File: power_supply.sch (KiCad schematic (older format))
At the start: 12 parts, among them IC704 TPS82085, IC705 TPS82085

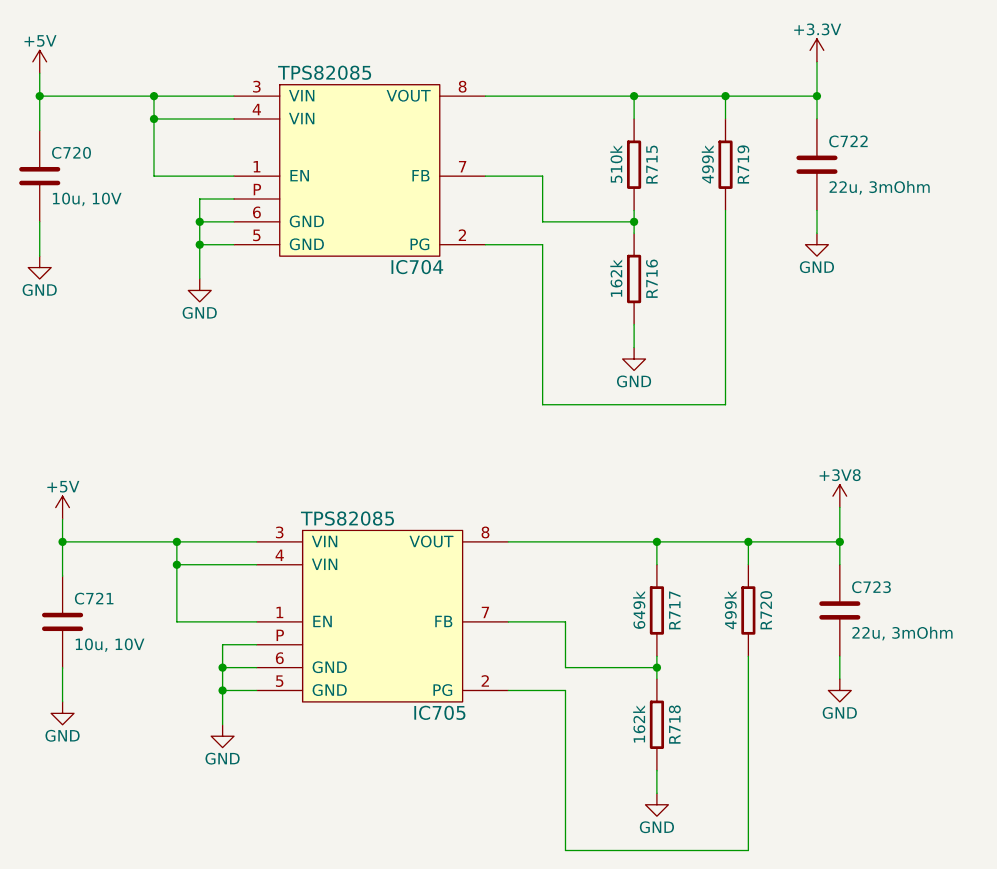
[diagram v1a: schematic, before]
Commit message: power Sypply for Tobyfinish
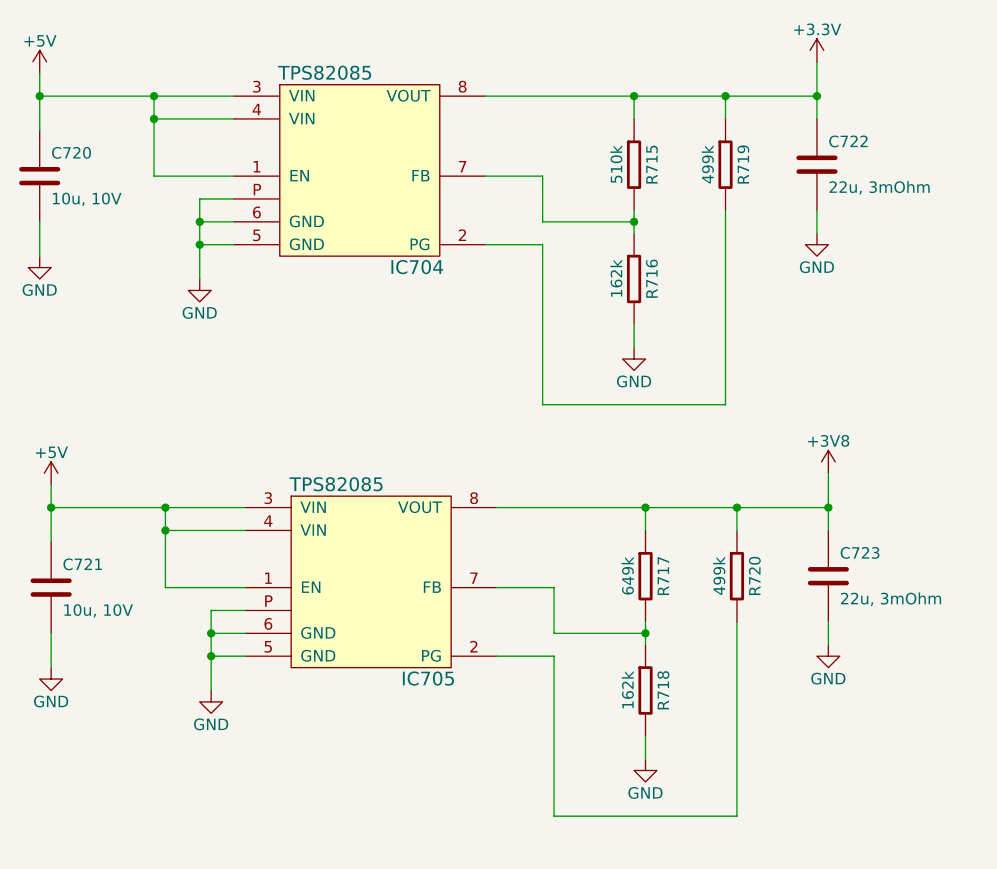
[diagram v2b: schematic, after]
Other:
- moved on the sheet: C721, C723, IC705, R717, R718, R720
